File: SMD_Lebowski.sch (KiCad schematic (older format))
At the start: 43 parts, among them U1 PIC30F4011

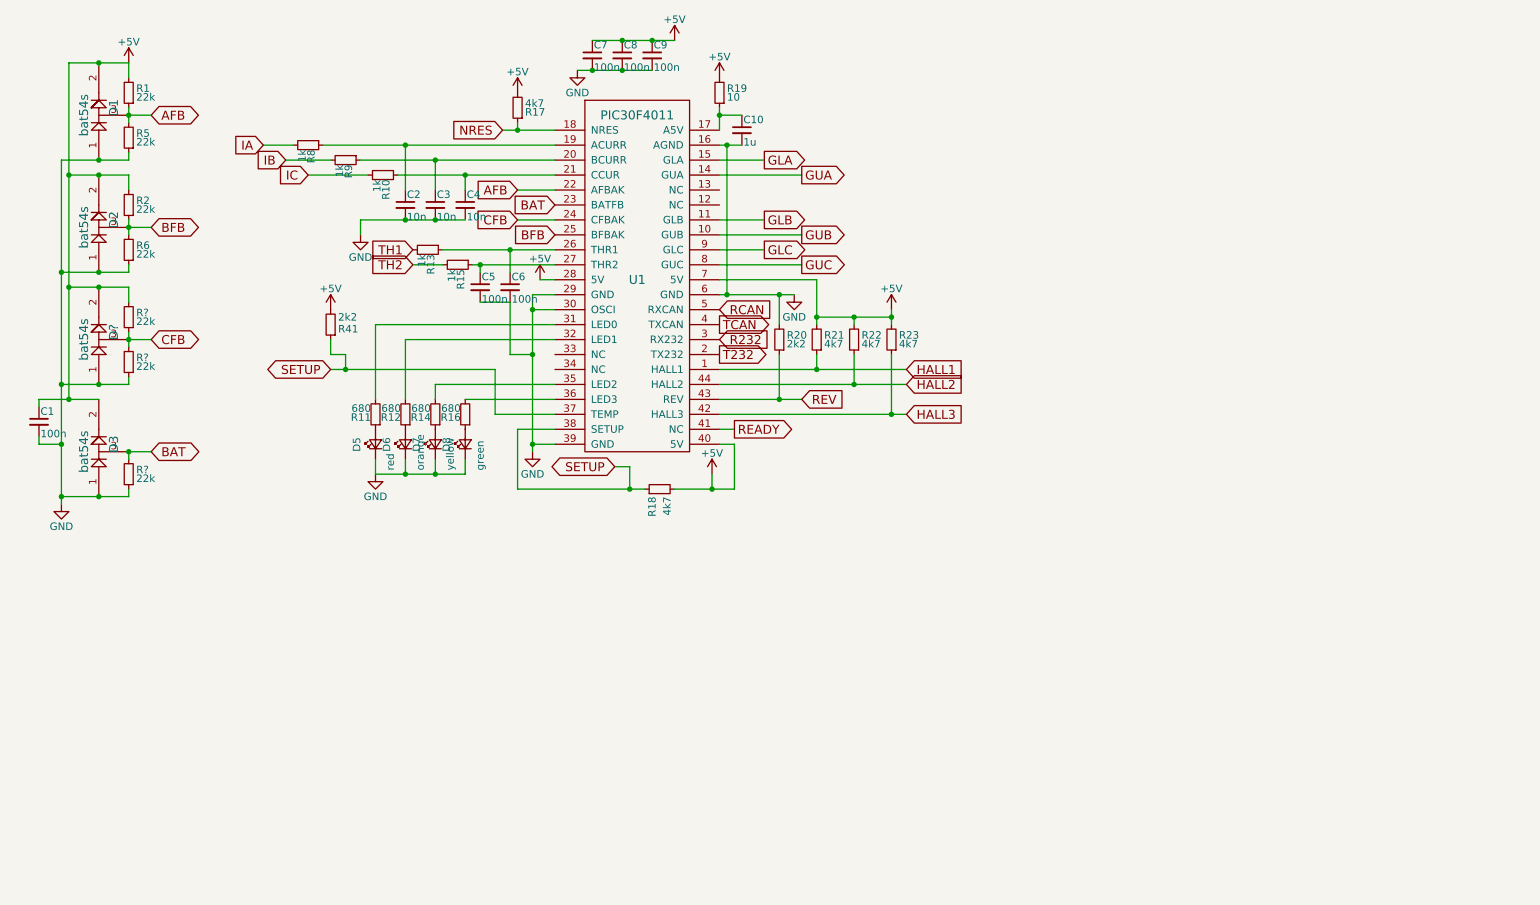
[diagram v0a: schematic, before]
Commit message: finished sc
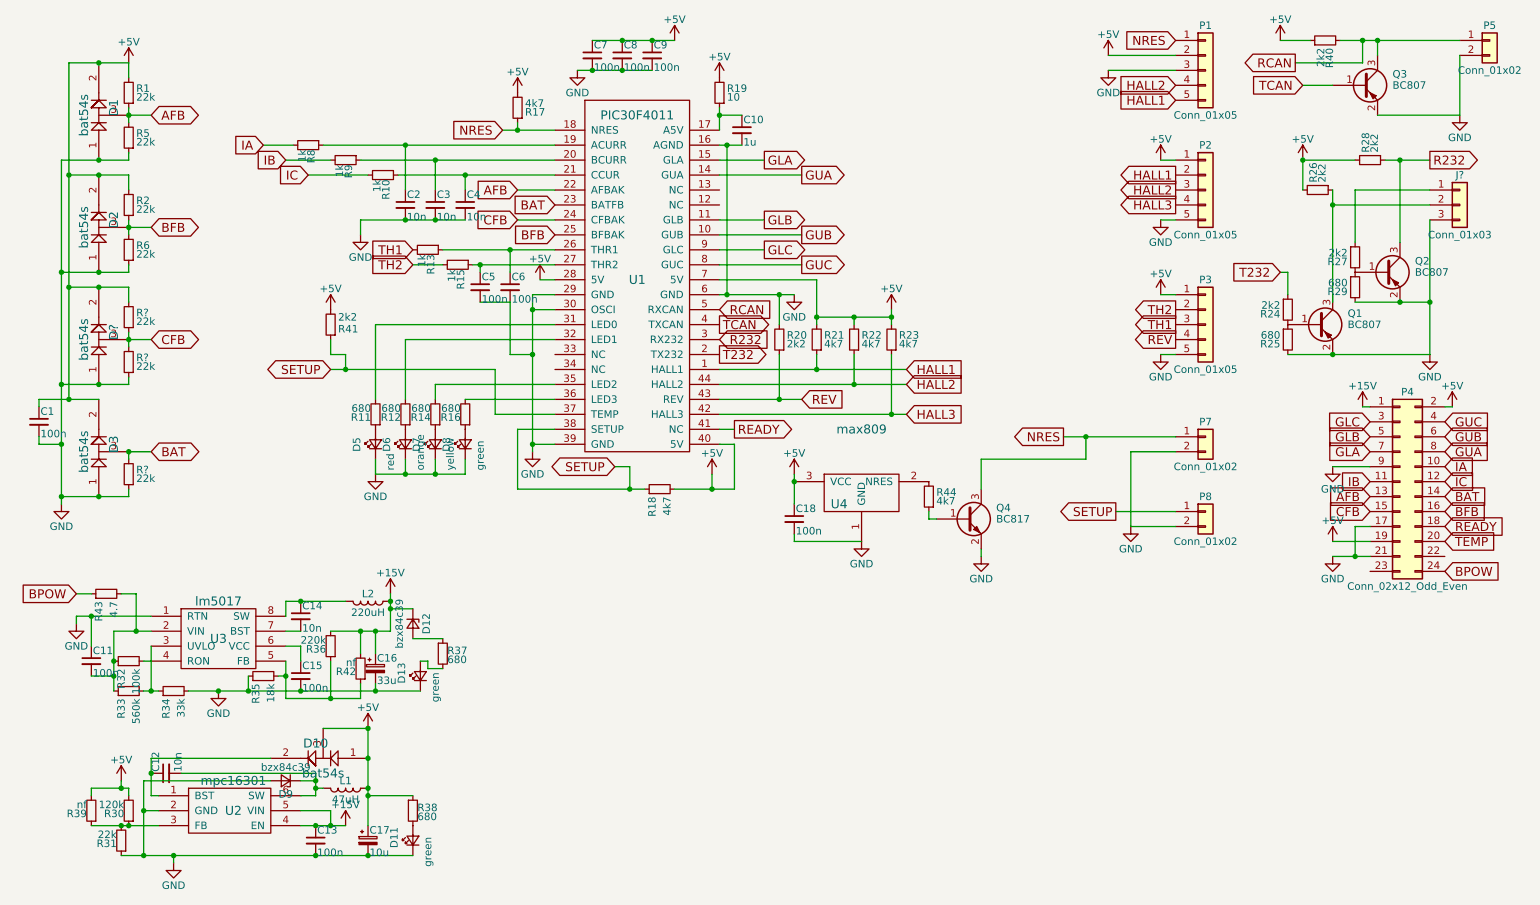
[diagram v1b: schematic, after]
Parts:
- added C11, C13, C15, C18: 100n, symbol C_Small
- added C12, C14: 10n, symbol C_Small
- added C16: 33u, symbol CP_Small
- added C17: 10u, symbol CP_Small
- added D10: bat54s, symbol bat54s
- added D11, D13: green, symbol LED_Small
- added D12, D9: bzx84c39, symbol bzx84c39
- added J?: Conn_01x03, symbol Conn_01x03
- added L1: 47uH, symbol L
- added L2: 220uH, symbol L
- added P1, P2, P3: Conn_01x05, symbol Conn_01x05
- added P4: Conn_02x12_Odd_Even, symbol Conn_02x12_Odd_Even
- added P5, P7, P8: Conn_01x02, symbol Conn_01x02
- added Q1, Q2, Q3: BC807, TO_SOT_Packages_SMD:SOT-23, symbol BC807
- added Q4: BC817, TO_SOT_Packages_SMD:SOT-23, symbol BC817
- added R24, R26, R27, R28, R40: 2k2, symbol R_Small
- added R25, R29, R37, R38: 680, symbol R_Small
- added R30: 120k, symbol R_Small
- added R31: 22k, symbol R_Small
- added R32: 100k, symbol R_Small
- added R33: 560k, symbol R_Small
- added R34: 33k, symbol R_Small
- added R35: 18k, symbol R_Small
- added R36: 220k, symbol R_Small
- added R39, R42: nf, symbol R_Small
- added R43: 4.7, symbol R_Small
- added R44: 4k7, symbol R_Small
- added U2: mpc16301, symbol mpc16301
- added U3: lm5017, symbol lm5017
- added U4: max809, symbol max809
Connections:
- net +5V: now also C17.1, C18.1, D10.1, D10.3, L1.1, P1.2 (Pin_2), P2.1 (Pin_1), P3.1 (Pin_1), P4.19 (Pin_19), P4.2 (Pin_2), R26.2, R28.2, R30.2, R38.1, R39.2, R40.1, U4.3 (VCC)
- net AFB: now also P4.13 (Pin_13)
- net BAT: now also P4.14 (Pin_14)
- net BFB: now also P4.16 (Pin_16)
- net CFB: now also P4.15 (Pin_15)
- net GLA: now also P4.7 (Pin_7)
- net GLB: now also P4.5 (Pin_5)
- net GLC: now also P4.3 (Pin_3)
- net GND: now also C11.1, C13.2, C15.2, C16.2, C17.2, C18.2, D11.1 (K), D13.1 (K), D9.2 (A), J?.3 (Pin_3), P1.3 (Pin_3), P2.5 (Pin_5), P3.5 (Pin_5), P4.17 (Pin_17), P4.21 (Pin_21), P4.9 (Pin_9), P5.2 (Pin_2), P7.2 (Pin_2), P8.2 (Pin_2), Q1.2 (E), Q2.2 (E), Q3.2 (E), Q4.2 (E), R25.2, R29.2, R31.1, R34.2, R35.1, U2.2 (GND), U3.1 (RTN), U4.1 (GND)
- net GUA: now also P4.8 (Pin_8)
- net GUB: now also P4.6 (Pin_6)
- net GUC: now also P4.4 (Pin_4)
- net HALL1: now also P1.5 (Pin_5), P2.2 (Pin_2)
- net HALL2: now also P1.4 (Pin_4), P2.3 (Pin_3)
- net HALL3: now also P2.4 (Pin_4)
- net IA: now also P4.10 (Pin_10)
- net IB: now also P4.11 (Pin_11)
- net IC: now also P4.12 (Pin_12)
- net NRES: now also P1.1 (Pin_1), P7.1 (Pin_1), Q4.3 (C)
- net R232: now also Q2.3 (C), R28.1
- net RCAN: now also P5.1 (Pin_1), Q3.3 (C), R40.2
- net READY: now also P4.18 (Pin_18)
- net REV: now also P3.4 (Pin_4)
- net SETUP: now also P8.1 (Pin_1)
- net T232: now also R24.1
- net TCAN: now also Q3.1 (B)
- net TH1: now also P3.3 (Pin_3)
- net TH2: now also P3.2 (Pin_2)
- new net: Q4.1 (B), R44.1
- new net: R44.2, U4.2 (NRES)
- new net: Q1.1 (B), R24.2, R25.1
- new net: Q2.1 (B), R27.2, R29.1
- new net: J?.1 (Pin_1), R27.1
- new net: J?.2 (Pin_2), R26.1
- new net: C11.2, R32.1, R33.1, R43.2, U3.2 (VIN)
- new net: R33.2, R34.1, U3.3 (UVLO)
- new net: R32.2, U3.4 (RON)
- new net: R35.2, R36.1, R42.1, U3.5 (FB)
- new net: C15.1, U3.6 (VCC)
- new net: C14.2, U3.7 (BST)
- new net: C14.1, L2.2, U3.8 (SW)
- new net: D12.2 (A), R37.1
- new net: D13.2 (A), R37.2
- new net: C12.1, D10.2, U2.1 (BST)
- new net: C12.2, D9.1 (K), L1.2, U2.6 (SW)
- new net: D11.2 (A), R38.2
- new net: R30.1, R31.2, R39.1, U2.3 (FB)
- new net +15V: C13.1, C16.1, D12.1 (K), L2.1, P4.1 (Pin_1), R36.2, R42.2, U2.4 (EN), U2.5 (VIN)
- new net BPOW: P4.24 (Pin_24), R43.1
- new net TEMP: P4.20 (Pin_20)

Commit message: Finished board layout
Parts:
- C1, C10, C11, C12, C13, C14, C15, C18, C2, C3, C4, C5, C6, C7, C8, C9: footprint (none) -> Capacitor_SMD:C_0805_2012Metric_Pad1.29x1.40mm_HandSolder
- C16: footprint (none) -> Capacitor_SMD:C_2816_7142Metric_Pad2.55x4.50mm_HandSolder
- C17: footprint (none) -> Capacitor_SMD:C_1210_3225Metric_Pad1.39x2.70mm_HandSolder
- D1, D2: footprint (none) -> Package_TO_SOT_SMD:SOT-23_Handsoldering
- D10, U4: footprint (none) -> Package_TO_SOT_SMD:SOT-23
- D11, D13, D5, D6, D7, D8: footprint (none) -> LED_SMD:LED_1206_3216Metric_Pad1.22x1.80mm_HandSolder
- D12: footprint (none) -> Package_TO_SOT_SMD:SOT-23_Handsoldering; symbol bzx84c39 -> bzx84c39-RESCUE-SMD_Lebowski
- D3: renamed from D?; footprint (none) -> Package_TO_SOT_SMD:SOT-23_Handsoldering
- D4: renamed from D3; footprint (none) -> Package_TO_SOT_SMD:SOT-23_Handsoldering
- D9: footprint (none) -> Package_TO_SOT_SMD:SOT-23; symbol bzx84c39 -> bzx84c39-RESCUE-SMD_Lebowski
- L1: footprint (none) -> Inductor_SMD:L_1210_3225Metric_Pad1.39x2.70mm_HandSolder
- L2: footprint (none) -> Inductor_SMD:L_10.4x10.4_H4.8
- P1, P2, P3: footprint (none) -> Connector_PinHeader_2.54mm:PinHeader_1x05_P2.54mm_Vertical
- P4: footprint (none) -> Connector_PinHeader_2.54mm:PinHeader_2x12_P2.54mm_Vertical
- P5, P7, P8: footprint (none) -> Connector_PinHeader_2.54mm:PinHeader_1x02_P2.54mm_Vertical
- P6: renamed from J?; footprint (none) -> Connector_PinHeader_2.54mm:PinHeader_1x04_P2.54mm_Vertical
- R1, R10, R11, R12, R13, R14, R15, R16, R17, R18, R19, R2, R20, R21, R22, R23, R24, R25, R5, R6, R8, R9: footprint (none) -> Resistor_SMD:R_0805_2012Metric_Pad1.29x1.40mm_HandSolder
- R26, R27, R28, R29, R30, R31, R32, R33, R34, R35, R36, R37, R38, R39, R40, R41, R42, R43, R44: footprint (none) -> Resistor_SMD:R_0815_2038Metric
- R3, R4, R7: renamed from R?; footprint (none) -> Resistor_SMD:R_0805_2012Metric_Pad1.29x1.40mm_HandSolder
- U1: footprint (none) -> Package_QFP:TQFP-44_10x10mm_P0.8mm
- U2: footprint (none) -> Package_TO_SOT_SMD:SOT-23-6_Handsoldering
- U3: footprint (none) -> Package_SO:SOIC-8_3.9x4.9mm_P1.27mm
